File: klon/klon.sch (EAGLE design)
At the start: 14 parts, among them IC1 MAX1044

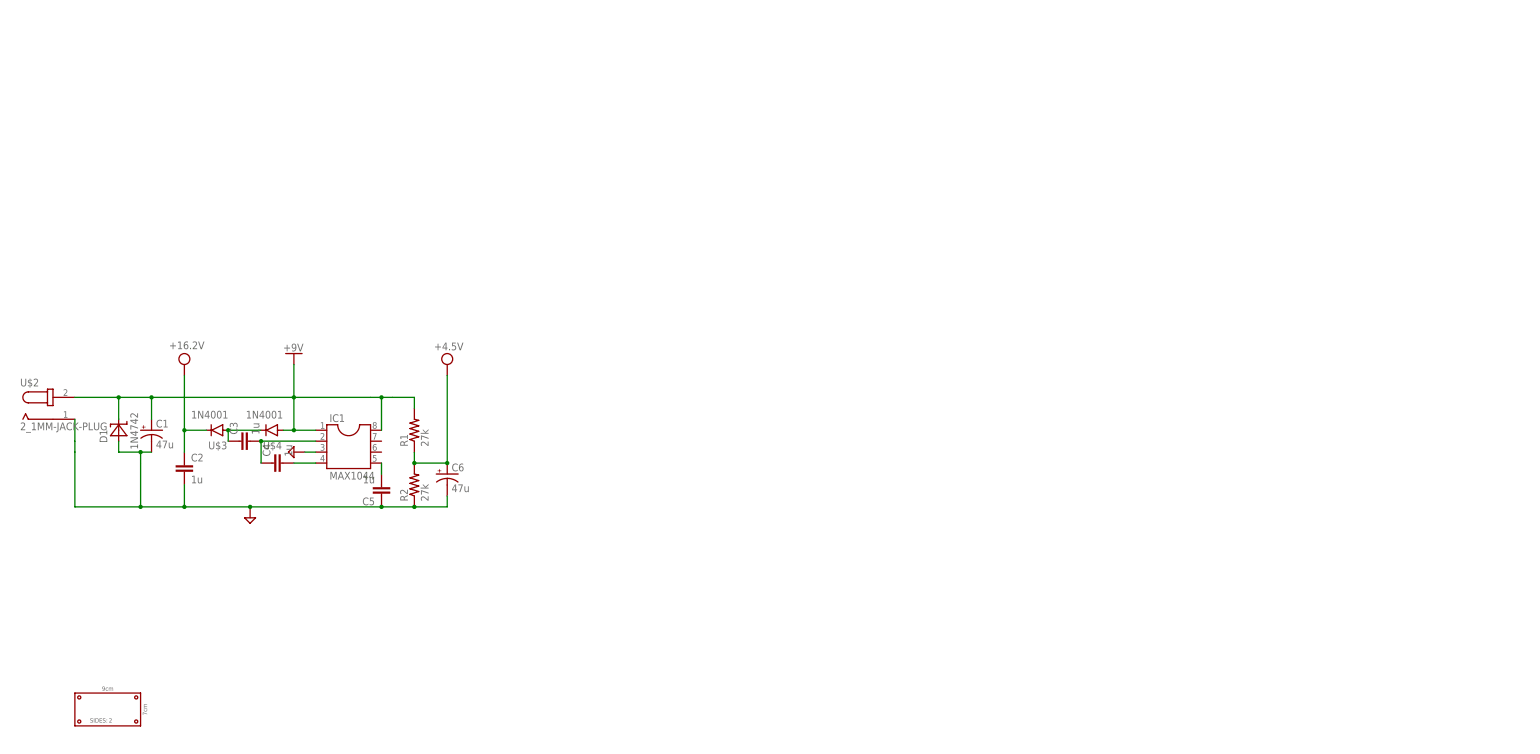
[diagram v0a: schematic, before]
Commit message: Klon schematic
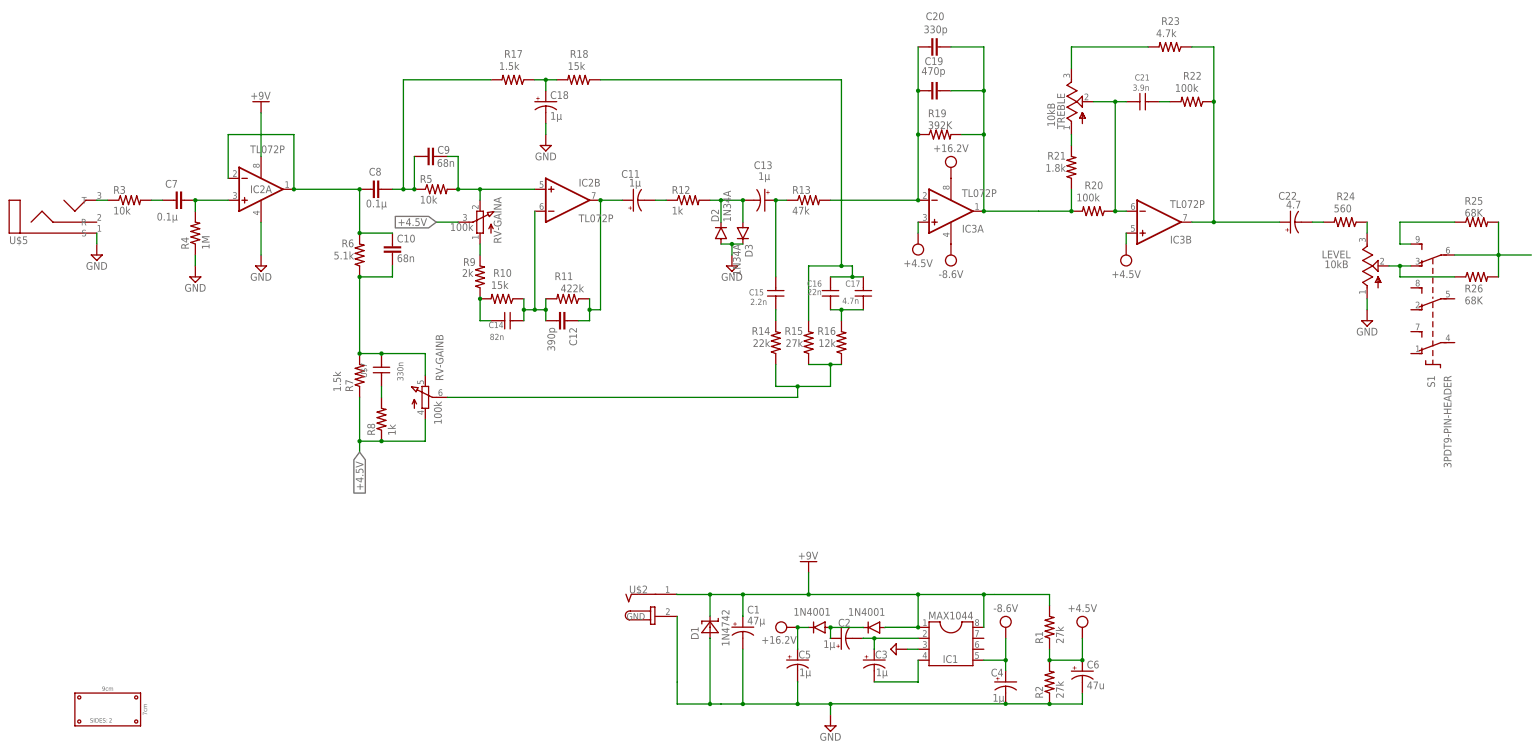
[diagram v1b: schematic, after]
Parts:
- added C10, C9: 68n, capacitor-wima:C10/5
- added C11, C13, C18: 1µ, pedal-library:C-E0.1_0.15
- added C12: 390p, pedal-library:C-CERAMICC-C-0.1_0.05
- added C14: 82n, pedal-library:C-PP_0.60.2W
- added C15: 2.2n, pedal-library:C-PP_0.40.15
- added C16: 22n, pedal-library:C-PP_0.40.2
- added C17: 4.7n, pedal-library:C-PP_0.40.2
- added C19: 470p, pedal-library:C-CERAMICC-C-0.1_0.05
- added C20: 330p, pedal-library:C-CERAMICC-C-0.1_0.05
- added C21: 3.9n, pedal-library:C-PP_0.40.1
- added C22: 4.7, pedal-library:C-E0.1_0.15
- added C7, C8: 0.1µ, capacitor-wima:C10/5
- added D2, D3: 1N34A, diode:DIODE-D-7.5
- added IC2, IC3: TL072P, linear:TL072P
- added LEVEL, TREBLE: 10kB, pedal-library:POT-1X
- added R10, R18: 15k, pedal-library:RESISTOR0204/7
- added R11: 422k, pedal-library:RESISTOR0204/7
- added R12, R8: 1k, pedal-library:RESISTOR0204/7
- added R13: 47k, pedal-library:RESISTOR0204/7
- added R14: 22k, pedal-library:RESISTOR0204/7
- added R15: 27k, pedal-library:RESISTOR0204/7
- added R16: 12k, pedal-library:RESISTOR0204/7
- added R17, R7: 1.5k, pedal-library:RESISTOR0204/7
- added R19: 392K, pedal-library:RESISTOR0204/7
- added R20, R22: 100k, pedal-library:RESISTOR0204/7
- added R21: 1.8k, pedal-library:RESISTOR0204/7
- added R23: 4.7k, pedal-library:RESISTOR0204/7
- added R24: 560, pedal-library:RESISTOR0204/7
- added R25, R26: 68K, pedal-library:RESISTOR0204/7
- added R3, R5: 10k, pedal-library:RESISTOR0204/7
- added R4: 1M, pedal-library:RESISTOR0204/7
- added R6: 5.1k, pedal-library:RESISTOR0204/7
- added R9: 2k, pedal-library:RESISTOR0204/7
- added RV-GAIN: 100k, pedal-library:POT-2X
- added S1: 3PDT9-PIN-HEADER, pedal-library:3PDT9-PIN-HEADER
- added U$5: INSTRUMENT-JACKPINS, pedal-library:INSTRUMENT-JACKPINS
- added U$7: 330n, pedal-library:C-PP_0.60.15W
- C1: value 47u -> 47µ
- C2, C3, C4, C5: value 1u -> 1µ; device pedal-library:C-MM025-025X050 -> pedal-library:C-E0.1_0.15
- U$1: value (none) -> 9x7
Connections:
- new net -8.6V: C4.+, IC1.5, IC3P.V-
- new net N$1: C2.-, C3.+, IC1.2
- new net N$10: C10.2, C8.1, IC2A.-IN, IC2A.OUT, R6.2
- new net N$11: C10.1, R6.1, R7.2, RV-GAINB.E, U$7.2
- new net N$12: R9.2, RV-GAINA.A
- new net N$13: C14.1, R10.2, R9.1
- new net N$14: C11.-, R12.1
- new net N$15: C13.-, D2.C, D3.A, R12.2
- new net N$16: C11.+, C12.1, IC2B.OUT, R11.1
- new net N$17: C12.2, C14.2, IC2B.-IN, R10.1, R11.2
- new net N$18: C13.+, C15.2, R13.1
- new net N$19: C15.1, R14.2
- new net N$20: R14.1, R15.1, R16.1, RV-GAINB.S
- new net N$21: C16.1, C17.1, R16.2
- new net N$22: C16.2, C17.2, R15.2, R18.1
- new net N$23: C18.+, R17.1, R18.2
- new net N$24: R21.2, TREBLE.1
- new net N$25: C19.2, C20.2, IC3A.OUT, R19.2, R20.2, R21.1
- new net N$26: C19.1, C20.1, IC3A.-IN, R13.2, R19.1
- new net N$27: C21.1, IC3B.-IN, R20.1, TREBLE.2
- new net N$28: C22.+, IC3B.OUT, R22.1, R23.1
- new net N$29: R23.2, TREBLE.3
- new net N$30: C21.2, R22.2
- new net N$31: C22.-, R24.2
- new net N$32: LEVEL.3, R24.1
- new net N$33: LEVEL.2, R26.1, S1.O3
- new net N$34: R25.1, S1.S3
- new net N$35: R25.2, R26.2, S1.P3
- new net N$4: C2.+, U$3.A, U$4.C
- new net N$7: R8.2, U$7.1
- new net N$8: C8.2, C9.1, R17.2, R5.1
- new net N$9: C9.2, IC2B.+IN, R5.2, RV-GAINA.E
- net +16.2V: now also C5.+, IC3P.V+; no longer C2.1
- net +4.5V: now also IC3A.+IN, IC3B.+IN, R7.1, R8.1, RV-GAINA.S, RV-GAINB.A
- net +9V: now also IC2P.V+, U$2.+9V; no longer U$2.GND
- net GND: now also C18.-, C4.-, C5.-, D2.A, D3.C, IC2P.V-, LEVEL.1, R4.1, U$2.GND, U$5.S; no longer C2.2, C5.1, U$2.+9V
- net N$2: now also C3.-, IC1.4; no longer C5.2, IC1.5
- net N$3: now also C7.1, R3.2; no longer C3.1, U$3.A, U$4.C
- net N$5: now also R3.1, U$5.T; no longer C4.2, IC1.4
- net N$6: now also C7.2, IC2A.+IN, R4.2; no longer C3.2, C4.1, IC1.2
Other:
- moved on the sheet: C1, C6, D1, IC1, R1, R2
